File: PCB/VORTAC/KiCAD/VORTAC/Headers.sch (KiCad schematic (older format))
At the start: 20 parts, among them J1 MillMax_004, J10 FAN_01_V, J11 STEPPER, J12 IO, J13 918-418K2023S40001, J14 FAN_02_V, J15 LED_V, J16 THERM_R, J2 MillMax_004, J3 DEBUG, J4 USB_HOST, J5 FAN_01, J6 FAN_02, J7 LED, J8 HOTEND, J9 Conn_02x03_Odd_Even

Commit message: progress
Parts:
- added D5: D_Schottky, symbol Device:D_Schottky
- added H1, H2: M3, MountingHole:MountingHole_3mm_Pad_Via, symbol Mechanical:MountingHole_Pad
- added JP1, JP2: SolderJumper_2_Bridged, ToolChanger:SolderJumper_Hex_Bridged_Pad, symbol Jumper:SolderJumper_2_Bridged
- added JP3, JP4: SolderJumper_2_Open, ToolChanger:SolderJumper_Hex_Open_Pad, symbol Jumper:SolderJumper_2_Open
- J2: renamed from J9; value Conn_02x03_Odd_Even -> Molex Micro Fit 3.0; symbol Connector_Generic:Conn_02x03_Odd_Even -> Connector_Generic:Conn_02x03_Top_Bottom
- J6: renamed from J8; symbol Connector_Generic:Conn_02x02_Odd_Even -> Connector_Generic:Conn_02x02_Top_Bottom
- renumbered J3 to J1, J14 to J11, J15 to J12, J16 to J13, J13 to J14, J11 to J15, J12 to J16, J1 to J3, J2 to J4, J4 to J5, J5 to J7, J6 to J8, J7 to J9, R3 to R1, R4 to R2, R1 to R3, R2 to R4
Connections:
- net labels added: HOST_USB_D+, HOST_USB_D-, HOST_USB_DRAIN, THERM_1_OUT, TOOL_DATA_H, TOOL_DATA_L, USB_D+, USB_D-
- net labels removed: ???, HOST_D+, HOST_D-, THERM_1, USBH_D+, USBH_D-, USBH_DRAIN, USBMCU_D+, USBMCU_D-
- no-connect marks 4 -> 3
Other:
- note added: "Debug Header"
- note added: "Host USB Header"
- note added: "Uplink USB Port \nfor nozzlecams"
- note removed: "Debug & Programmin Header"
- note removed: "USB Uplink Header"
- moved on the sheet: J1, J10, J11, J12, J13, J14, J15, J16, J2, J3, J4, J5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

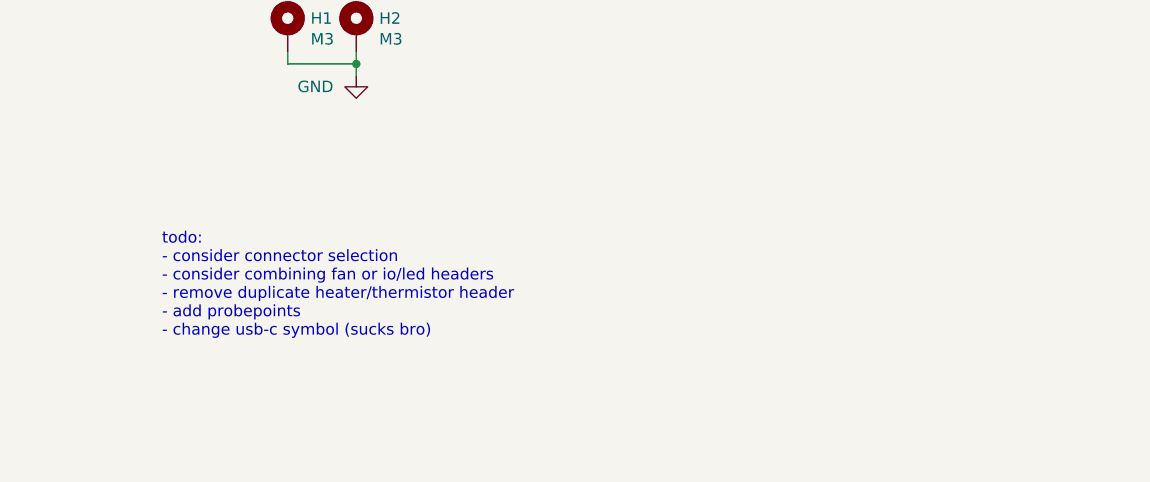
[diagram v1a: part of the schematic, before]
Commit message: progress
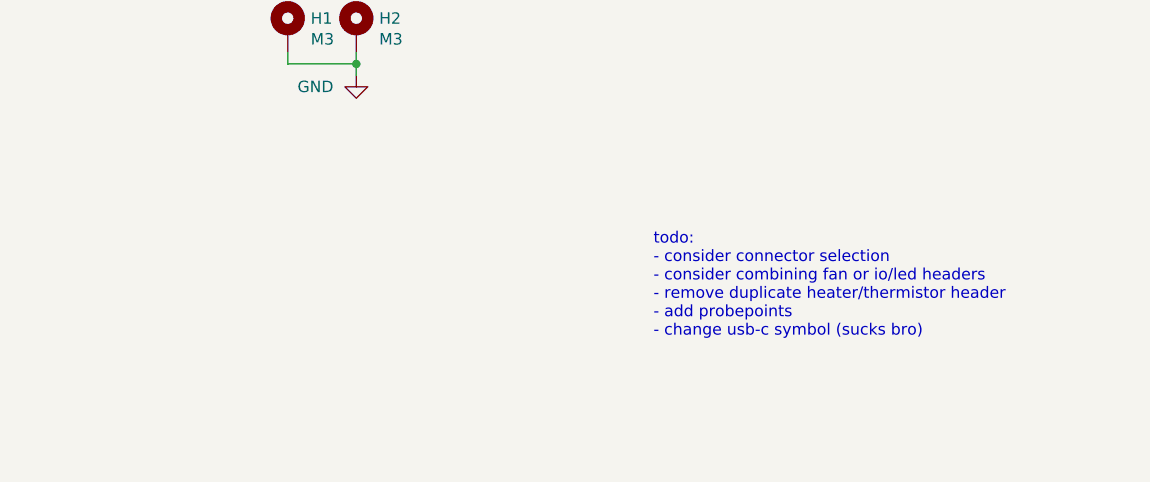
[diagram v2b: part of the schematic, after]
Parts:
- D5: footprint (none) -> Diode_SMD:D_SOD-123; LCSC (none) -> C37049
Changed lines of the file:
@@
 encoding utf-8
 Sheet 2 4
-Title ""
-Date ""
-Rev ""
-Comp ""
-Comment1 ""
-Comment2 ""
-Comment3 ""
-Comment4 ""
+Title "Headers & Tool Interfacing"
+Date "2021-10-17"
+Rev "0.0"
+Comp "VORTAC DESIGN"
+Comment1 "!! wip untested revesion !!"
+Comment2 "Designed to be used with Klipper Firmware"
+Comment3 "Canbus Networked Smart Tool Board"
+Comment4 "-- VORTAC PCB --"
 $EndDescr
 $Comp
@@
 Text Notes 3550 900  0    71   ~ 0
 Combined Hotend Header
-Text Notes 7050 7050 0    50   ~ 0
+Text Notes 9200 7050 0    50   ~ 0
 todo:\n- consider connector selection\n- consider combining fan or io/led headers\n- remove duplicate heater/thermistor header\n- add probepoints\n- change usb-c symbol (sucks bro)
 NoConn ~ 1400 1350
@@
 F 0 "D5" H 2200 5733 50  0000 C CNN
 F 1 "D_Schottky" H 2200 5824 50  0000 C CNN
-F 2 "" H 2200 5950 50  0001 C CNN
-F 3 "~" H 2200 5950 50  0001 C CNN
+F 2 "Diode_SMD:D_SOD-123" H 2200 5950 50  0001 C CNN
+F 3 "https://www.lcsc.com/product-detail/Schottky-Barrier-Diodes-SBD_MDD-Microdiode-Electronics-DSK14_C37049.html" H 2200 5950 50  0001 C CNN
+F 4 "C37049" H 2200 5950 50  0001 C CNN "LCSC"
 	1    2200 5950
 	-1   0    0    1
